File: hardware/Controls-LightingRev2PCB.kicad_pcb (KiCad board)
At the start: 2 copper layers, 50 x 55.7 mm, 49 parts, among them IC1 LM74502HDDFR, IC3 ACS724LLCTR-05AU-T, IC4 ACS724LLCTR-05AU-T, IC5 TLV70433DBVT, IC6 ACS724LLCTR-05AU-T, J1 53307-2471, J2 MX150_02x08_RightAngle, Q1 NVMFWS1D7N04XMT1G, Q3 IRLML0030, Q4 NVMFWS1D7N04XMT1G, Q5 IRLML0030, U5 SN74LV1T34DBV

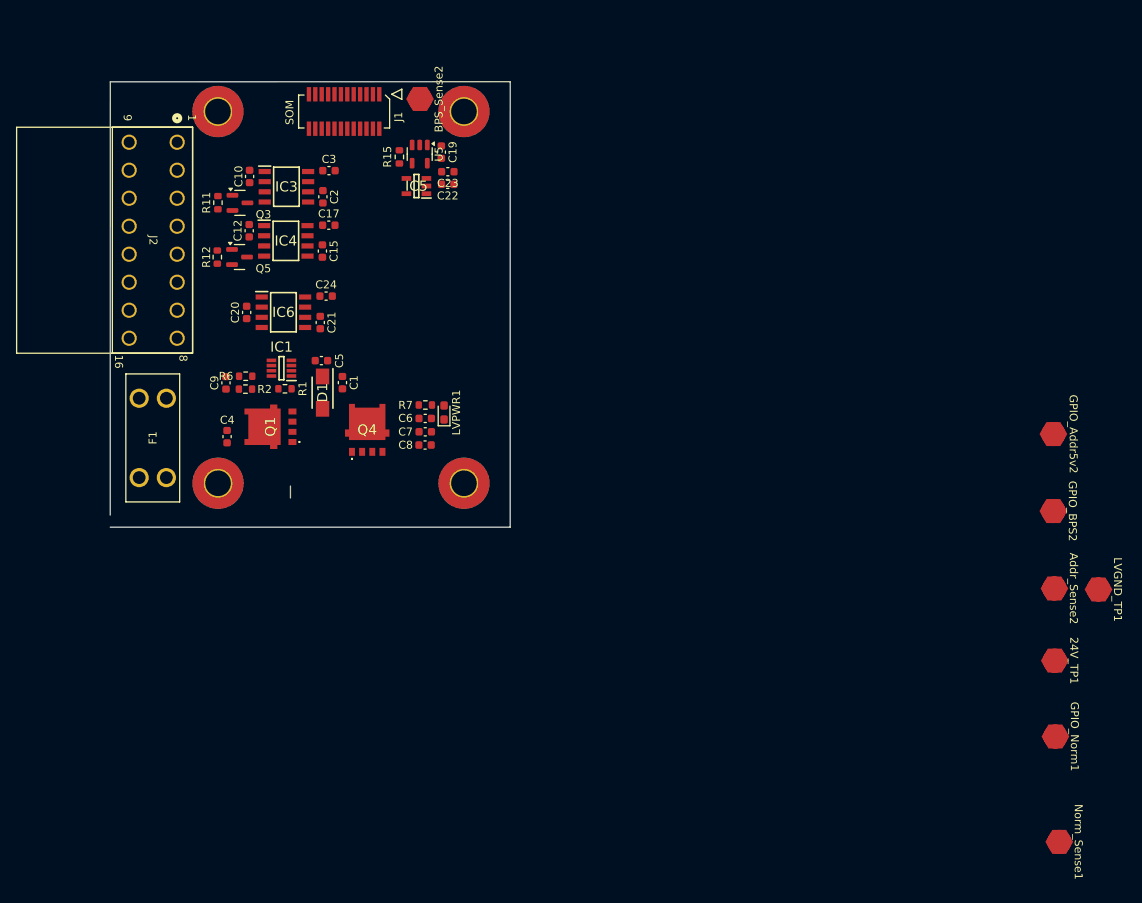
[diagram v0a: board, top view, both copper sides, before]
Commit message: Current Layout
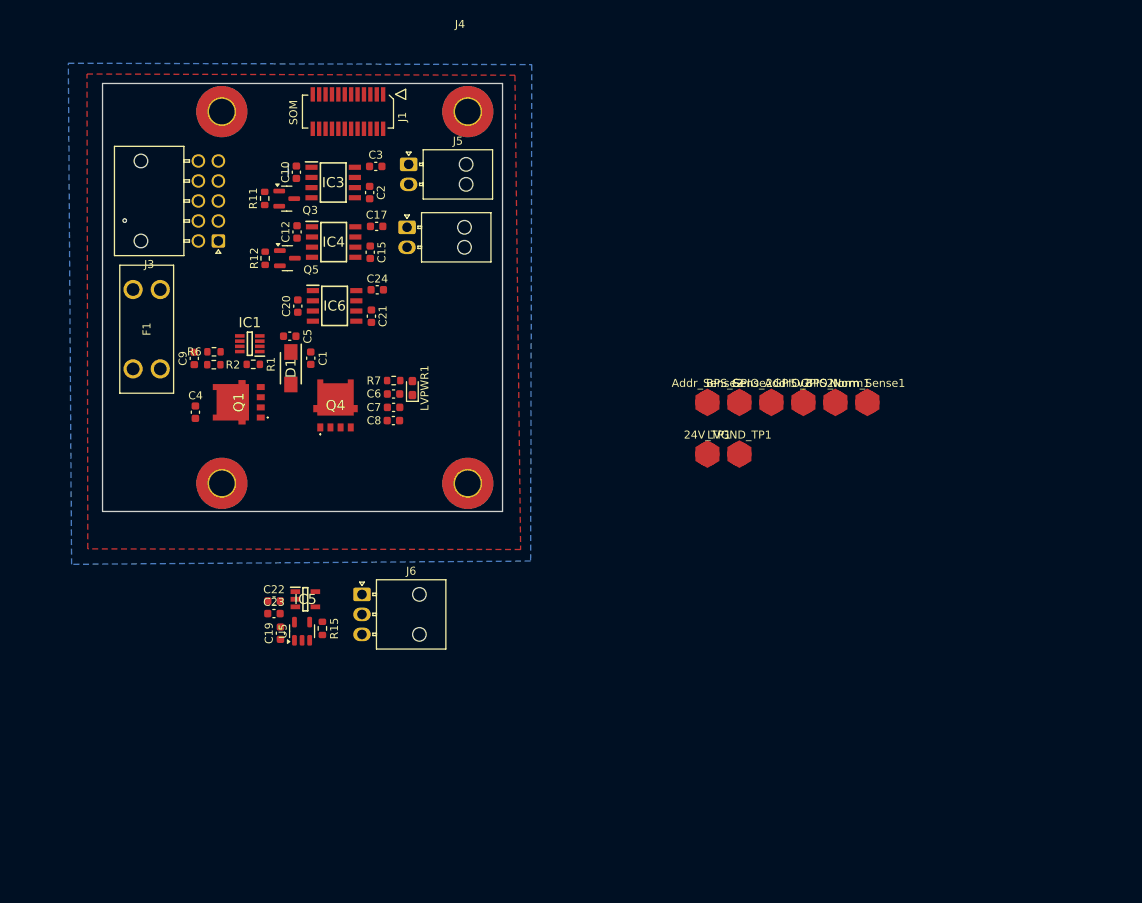
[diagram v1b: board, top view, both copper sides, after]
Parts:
- removed J2: MX150_02x08_RightAngle, UTSVT_Connectors:MX150_02x08_RightAngle
- added J3: Conn_02x05_Top_Bottom, Connector_Molex:Molex_Nano-Fit_105314-xx10_2x05_P2.50mm_Horizontal, F.Cu at (50.9, 39.8)
- added J4: Conn_01x02, UTSVT_Connectors:105313-2102, F.Cu at (74.5, 38.1)
- added J5: Conn_01x02, UTSVT_Connectors:105313-2102, F.Cu at (74.7, 30.2)
- added J6: Conn_01x03, UTSVT_Connectors:105313-1103, F.Cu at (68.8, 84.0)
- moved C19 63.4 mm to (58.6, 88.8), turned to 90 degrees
- moved U5 61.4 mm to (61.3, 88.6), turned to 90 degrees
- moved Norm_Sense1 59.9 mm to (132.0, 60.0), turned to 0 degrees
- moved R15 59.7 mm to (63.9, 88.3), turned to 90 degrees
- moved C23 59.4 mm to (57.8, 86.4), turned to 0 degrees
- moved C22 56.4 mm to (57.8, 84.8), turned to 0 degrees
- moved BPS_Sense2 55.1 mm to (116.0, 60.0), turned to 0 degrees
- moved IC5 53.5 mm to (61.7, 84.6), turned to 0 degrees
- moved 24V_TP1 50.5 mm to (112.0, 66.5), turned to 0 degrees
- moved GPIO_Norm1 50.0 mm to (128.0, 60.0), turned to 0 degrees
- moved Addr_Sense2 49.2 mm to (112.0, 60.0), turned to 0 degrees
- moved LVGND_TP1 48.0 mm to (116.0, 66.5), turned to 0 degrees
- moved GPIO_Addr5v2 35.5 mm to (120.0, 60.0), turned to 0 degrees
- moved GPIO_BPS2 34.1 mm to (124.0, 60.0), turned to 0 degrees
- moved F1 13.6 mm to (41.9, 50.9)
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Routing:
- net Addressable_GND: vias 0 -> 1
- added copper zone on B.Cu, net Addressable_GND
- added copper zone on F.Cu, net Addressable_PWR
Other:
- board size 50 x 55.7 mm -> 50 x 53.5 mm

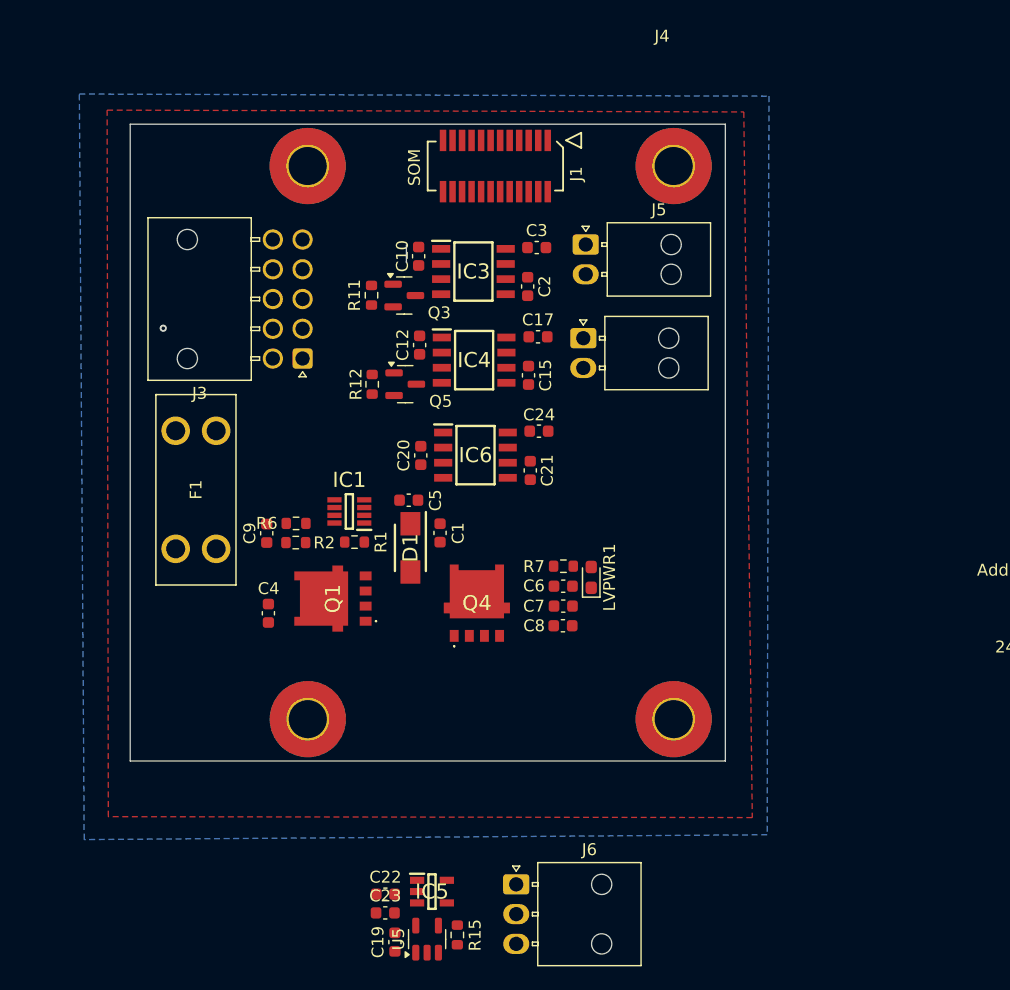
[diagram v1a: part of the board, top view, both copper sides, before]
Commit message: Layout
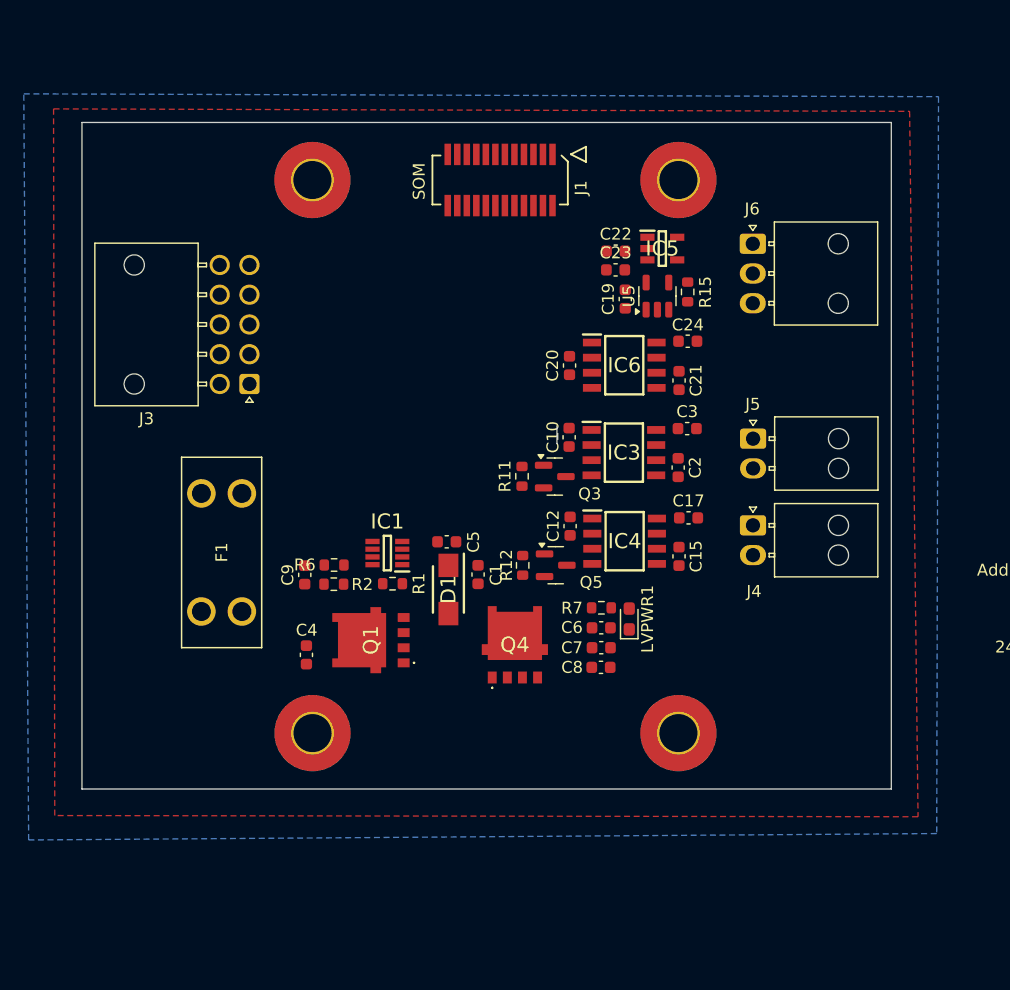
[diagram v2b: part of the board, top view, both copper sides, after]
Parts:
- moved C22 57.4 mm to (77.2, 30.8)
- moved U5 57.4 mm to (80.7, 34.6)
- moved C19 57.4 mm to (78.0, 34.8)
- moved C23 57.4 mm to (77.2, 32.4)
- moved R15 57.4 mm to (83.2, 34.2)
- moved IC5 57.4 mm to (81.1, 30.6)
- moved J6 57.4 mm to (88.7, 30.2)
- moved J5 21.5 mm to (88.7, 46.6)
- moved J4 21.2 mm to (88.7, 53.8)
- moved C10 19.8 mm to (73.3, 46.4)
- moved C15 19.8 mm to (82.5, 56.4)
- moved C17 19.8 mm to (83.3, 53.2)
- moved C2 19.8 mm to (82.4, 49.0)
- moved C3 19.8 mm to (83.2, 45.7)
- moved IC4 19.8 mm to (77.9, 55.2)
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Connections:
- J1 pad 11: BPS_Sense -> ADDR_Sense
- J1 pad 13: ADDR_Sense -> NORMAL_Sense
- J1 pad 15: NORMAL_Sense -> BPS_Sense
- J1 pad 17: GPIO_BPS_Strobe -> GPIO_Normal
- J1 pad 21: GPIO_Normal -> GPIO_BPS_Strobe
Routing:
- net Addressable_GND: vias 1 -> 0
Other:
- board size 50 x 53.5 mm -> 68 x 56 mm
